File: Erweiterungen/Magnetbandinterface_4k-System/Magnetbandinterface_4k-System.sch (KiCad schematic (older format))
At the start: 38 parts, among them T1 SC238d, T2 SC238, U17 B555D, U18 B761D, X13 DIN-3, X4 P3.6, X5 P3.0, X6 00, X7 BAS, X8 Video, X9 5V

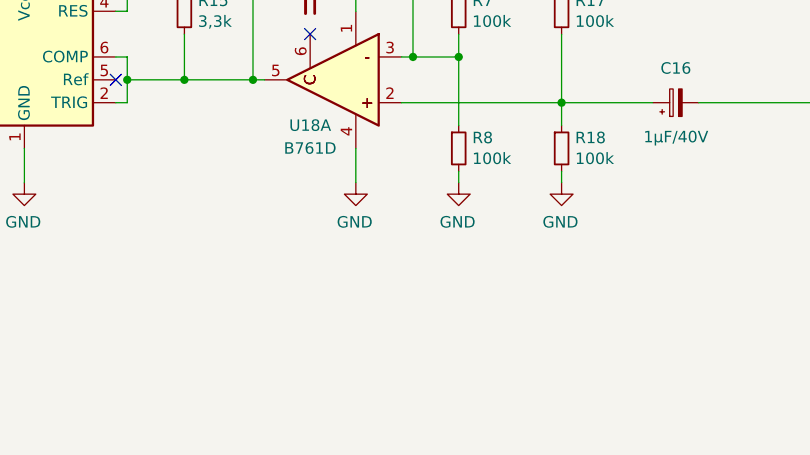
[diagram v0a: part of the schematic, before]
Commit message: Kommentar ergänzt
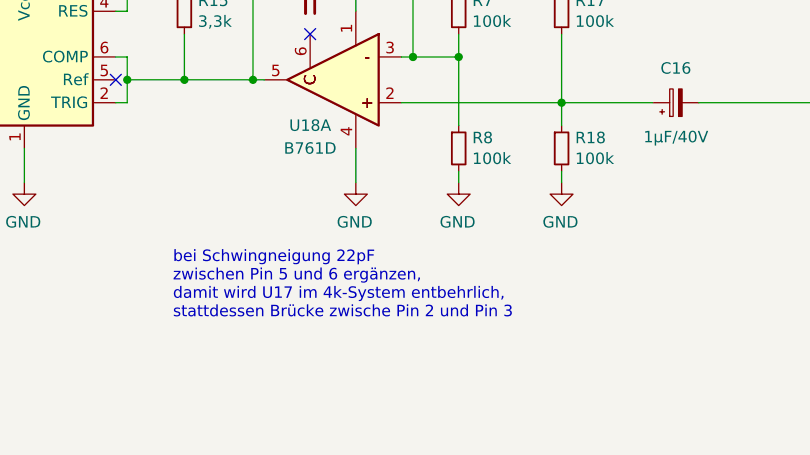
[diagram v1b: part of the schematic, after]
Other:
- note added: "bei Schwingneigung 22pF\nzwischen Pin 5 und 6 ergänzen,\ndamit wird U17 im 4k-System entbehrlich,\nstattdessen Brücke zwische Pin 2 und Pin 3"
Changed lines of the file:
@@
 	1    0    0    -1
 $EndComp
+Text Notes 5650 6500 0    50   ~ 0
+bei Schwingneigung 22pF\nzwischen Pin 5 und 6 ergänzen,\ndamit wird U17 im 4k-System entbehrlich,\nstattdessen Brücke zwische Pin 2 und Pin 3
 $EndSCHEMATC
